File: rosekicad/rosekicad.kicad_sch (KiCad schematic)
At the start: 78 parts, among them J1 Solenoid, J10 Solenoid, J11 Solenoid, J12 Solenoid, J13 UV Lights, J14 LED Lights, J15 DMX Cable, J16 Barrel_Jack_MountingPin, J2 Solenoid, J3 Solenoid, J4 Solenoid, J5 Solenoid, J6 Solenoid, J7 Solenoid, J8 Solenoid, J9 Solenoid, Q1 2N2222, Q10 2N2222, Q11 2N2222, Q12 2N2222, Q13 2N2222, Q14 2N2222, Q15 2N2222, Q2 2N2222, Q3 2N2222, Q4 2N2222, Q5 2N2222, Q6 2N2222, Q7 2N2222, Q8 2N2222, Q9 2N2222, U1 MAX485E

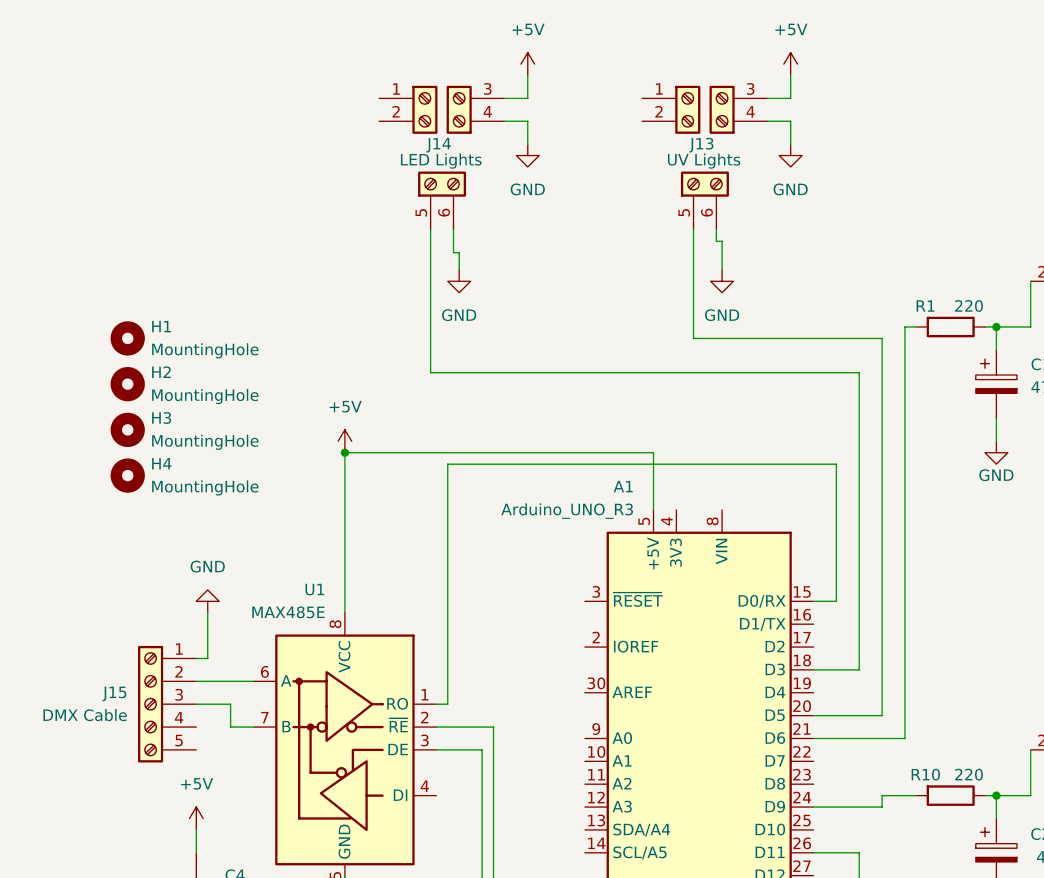
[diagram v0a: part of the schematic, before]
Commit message: final
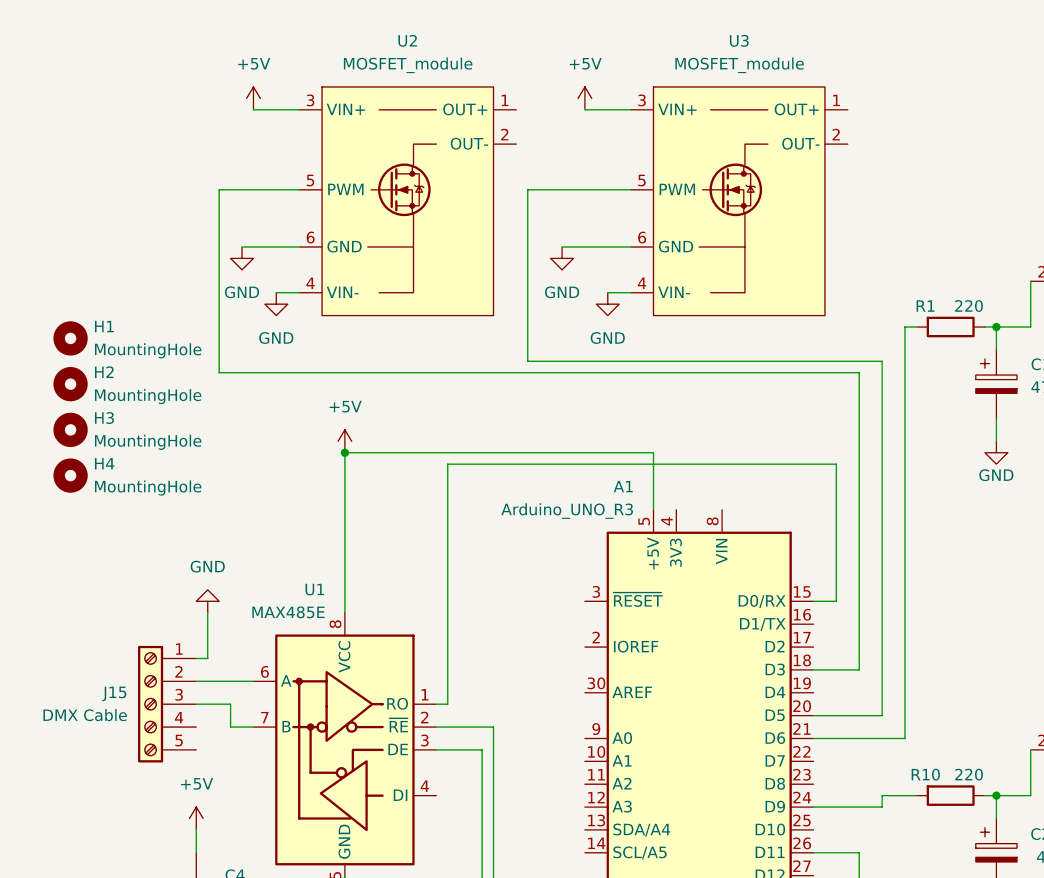
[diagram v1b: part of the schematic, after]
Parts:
- removed J13: UV Lights, rosekicad:MOSFET Switch Driver Module, symbol Connector:Screw_Terminal_01x02
- removed J14: LED Lights, rosekicad:MOSFET Switch Driver Module, symbol Connector:Screw_Terminal_01x02
- added U2, U3: MOSFET_module, rosekicad:MOSFET Switch Driver Module, symbol MOSFET_module:MOSFET_module
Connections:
- net +5V: now also U2.3 (VIN+), U3.3 (VIN+)
- net GND: now also U2.4 (VIN-), U2.6 (GND), U3.4 (VIN-), U3.6 (GND)
- net at A1.18 (D3): now also U2.5 (PWM)
- net at A1.20 (D5): now also U3.5 (PWM)
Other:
- moved on the sheet: H1, H2, H3, H4

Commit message: final
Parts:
- R11, R12, R13, R14, R2, R20, R21, R22, R23, R3, R4, R5: footprint Resistor_THT:R_Axial_DIN0207_L6.3mm_D2.5mm_P7.62mm_Horizontal -> Resistor_THT:R_Axial_DIN0414_L11.9mm_D4.5mm_P15.24mm_Horizontal
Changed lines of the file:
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@@
 			)
 		)
-		(property "Footprint" "Resistor_THT:R_Axial_DIN0207_L6.3mm_D2.5mm_P7.62mm_Horizontal"
+		(property "Footprint" "Resistor_THT:R_Axial_DIN0414_L11.9mm_D4.5mm_P15.24mm_Horizontal"
 			(at 143.002 133.35 90)
 			(effects
@@
 			)
 		)
-		(property "Footprint" "Resistor_THT:R_Axial_DIN0207_L6.3mm_D2.5mm_P7.62mm_Horizontal"
+		(property "Footprint" "Resistor_THT:R_Axial_DIN0414_L11.9mm_D4.5mm_P15.24mm_Horizontal"
 			(at 184.912 80.01 90)
 			(effects
@@
 			)
 		)
-		(property "Footprint" "Resistor_THT:R_Axial_DIN0207_L6.3mm_D2.5mm_P7.62mm_Horizontal"
+		(property "Footprint" "Resistor_THT:R_Axial_DIN0414_L11.9mm_D4.5mm_P15.24mm_Horizontal"
 			(at 144.272 80.01 90)
 			(effects
@@
 			)
 		)
-		(property "Footprint" "Resistor_THT:R_Axial_DIN0207_L6.3mm_D2.5mm_P7.62mm_Horizontal"
+		(property "Footprint" "Resistor_THT:R_Axial_DIN0414_L11.9mm_D4.5mm_P15.24mm_Horizontal"
 			(at 205.232 27.94 90)
 			(effects
@@
 			)
 		)
-		(property "Footprint" "Resistor_THT:R_Axial_DIN0207_L6.3mm_D2.5mm_P7.62mm_Horizontal"
+		(property "Footprint" "Resistor_THT:R_Axial_DIN0414_L11.9mm_D4.5mm_P15.24mm_Horizontal"
 			(at 164.592 80.01 90)
 			(effects
@@
 			)
 		)
-		(property "Footprint" "Resistor_THT:R_Axial_DIN0207_L6.3mm_D2.5mm_P7.62mm_Horizontal"
+		(property "Footprint" "Resistor_THT:R_Axial_DIN0414_L11.9mm_D4.5mm_P15.24mm_Horizontal"
 			(at 203.962 133.35 90)
 			(effects
@@
 			)
 		)
-		(property "Footprint" "Resistor_THT:R_Axial_DIN0207_L6.3mm_D2.5mm_P7.62mm_Horizontal"
+		(property "Footprint" "Resistor_THT:R_Axial_DIN0414_L11.9mm_D4.5mm_P15.24mm_Horizontal"
 			(at 183.642 133.35 90)
 			(effects
@@
 			)
 		)
-		(property "Footprint" "Resistor_THT:R_Axial_DIN0207_L6.3mm_D2.5mm_P7.62mm_Horizontal"
+		(property "Footprint" "Resistor_THT:R_Axial_DIN0414_L11.9mm_D4.5mm_P15.24mm_Horizontal"
 			(at 205.232 80.01 90)
 			(effects
@@
 			)
 		)
-		(property "Footprint" "Resistor_THT:R_Axial_DIN0207_L6.3mm_D2.5mm_P7.62mm_Horizontal"
+		(property "Footprint" "Resistor_THT:R_Axial_DIN0414_L11.9mm_D4.5mm_P15.24mm_Horizontal"
 			(at 163.322 133.35 90)
 			(effects
@@
 			)
 		)
-		(property "Footprint" "Resistor_THT:R_Axial_DIN0207_L6.3mm_D2.5mm_P7.62mm_Horizontal"
+		(property "Footprint" "Resistor_THT:R_Axial_DIN0414_L11.9mm_D4.5mm_P15.24mm_Horizontal"
 			(at 144.272 27.94 90)
 			(effects
@@
 			)
 		)
-		(property "Footprint" "Resistor_THT:R_Axial_DIN0207_L6.3mm_D2.5mm_P7.62mm_Horizontal"
+		(property "Footprint" "Resistor_THT:R_Axial_DIN0414_L11.9mm_D4.5mm_P15.24mm_Horizontal"
 			(at 164.592 27.94 90)
 			(effects
@@
 			)
 		)
-		(property "Footprint" "Resistor_THT:R_Axial_DIN0207_L6.3mm_D2.5mm_P7.62mm_Horizontal"
+		(property "Footprint" "Resistor_THT:R_Axial_DIN0414_L11.9mm_D4.5mm_P15.24mm_Horizontal"
 			(at 184.912 27.94 90)
 			(effects
